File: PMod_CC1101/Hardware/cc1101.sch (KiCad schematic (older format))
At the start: 17 parts

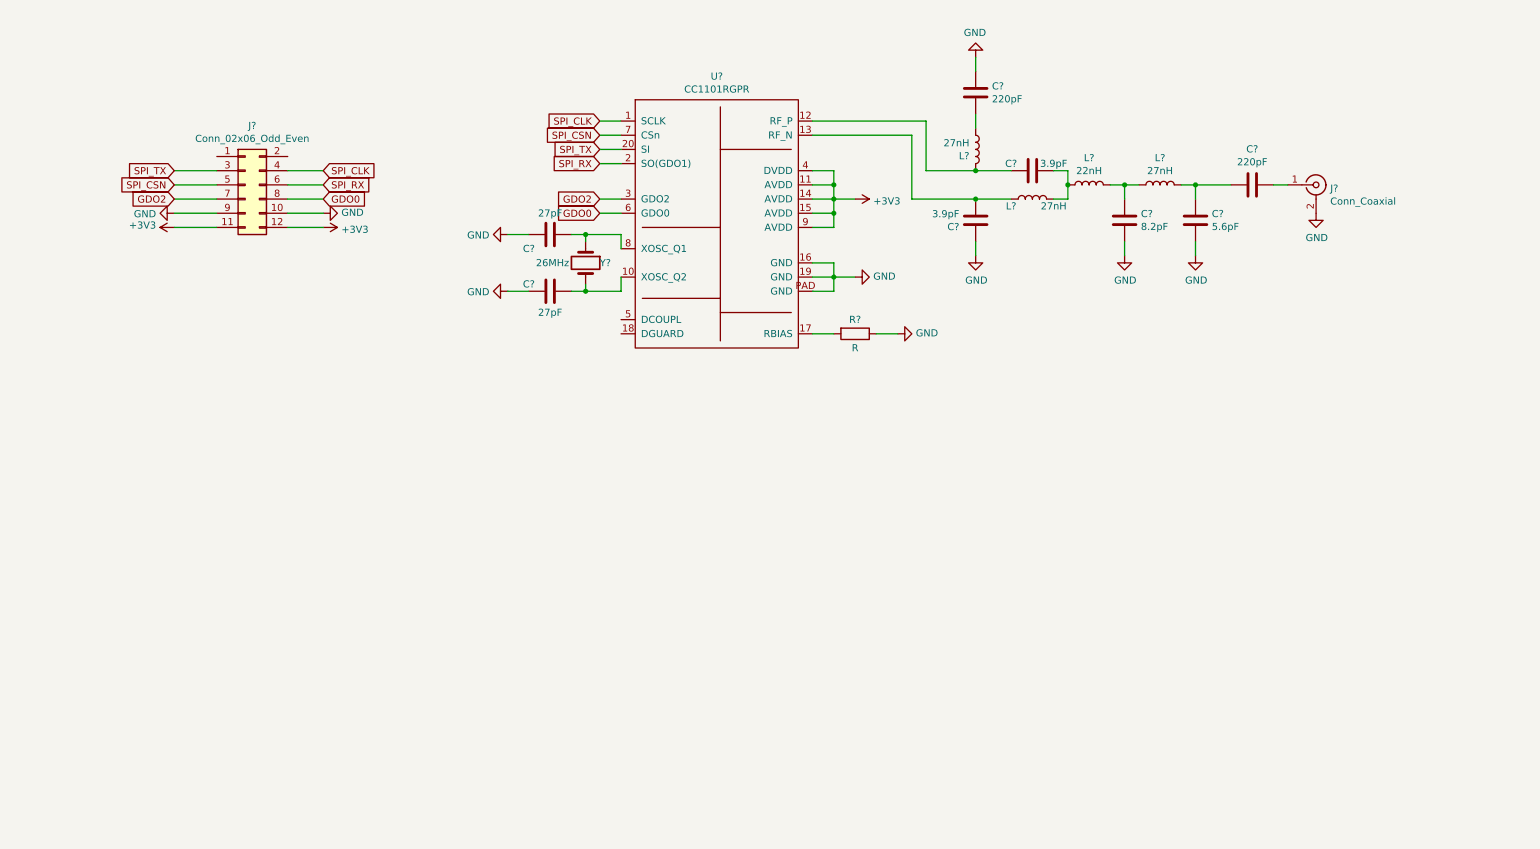
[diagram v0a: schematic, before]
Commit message: update the layout of the schematic
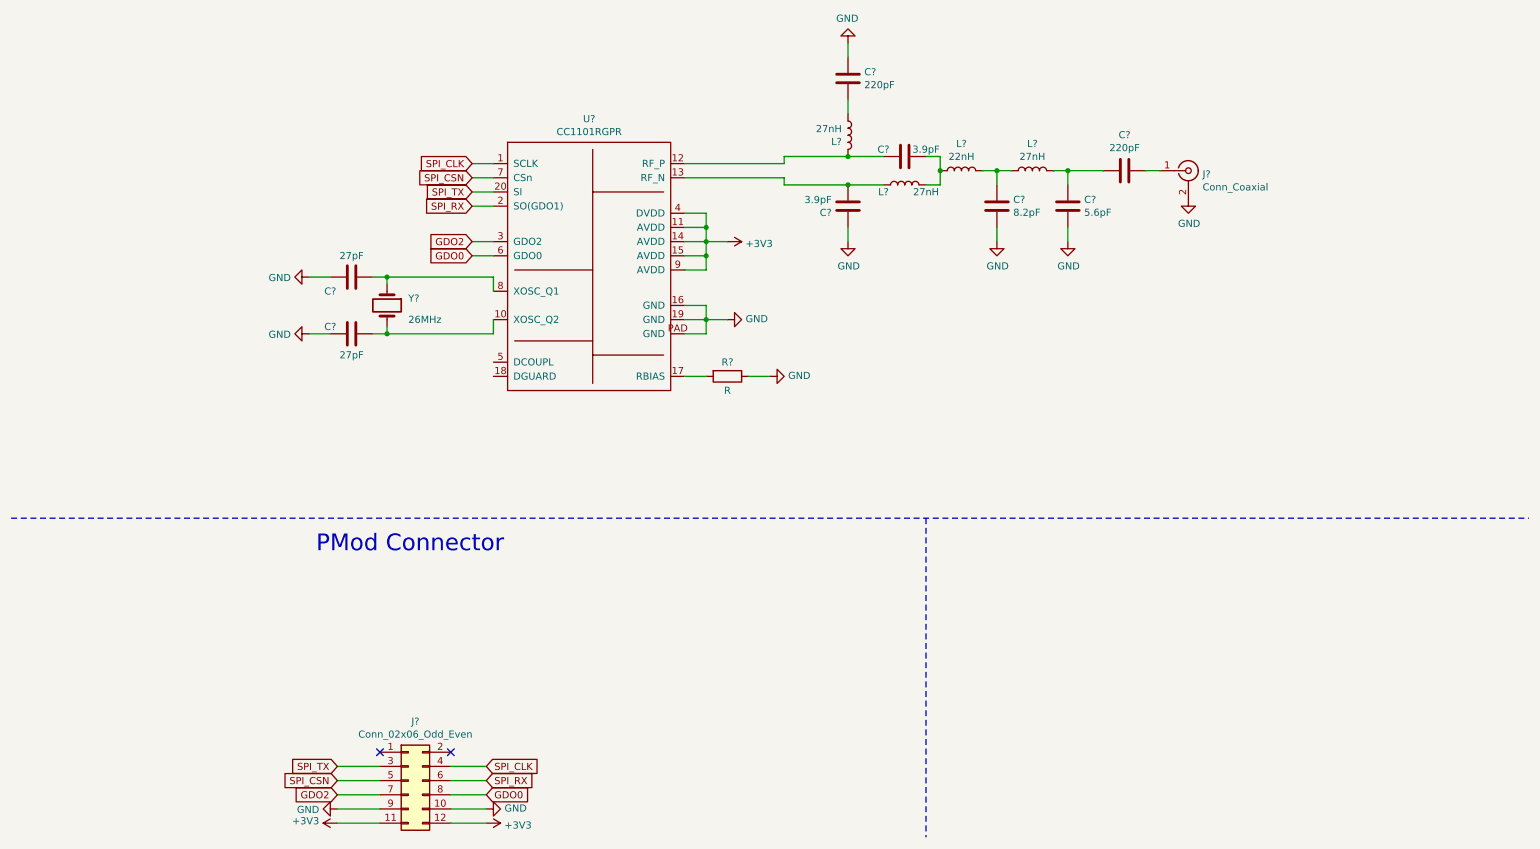
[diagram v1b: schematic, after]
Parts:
- J?: footprint (none) -> Connector_PinHeader_2.54mm:PinHeader_2x06_P2.54mm_Vertical
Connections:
- no-connect marks 0 -> 2
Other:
- note added: "PMod Connector"
- moved on the sheet: C?, J?, L?, R?, U?, Y?

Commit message: update the reference values and add a suitable crystal
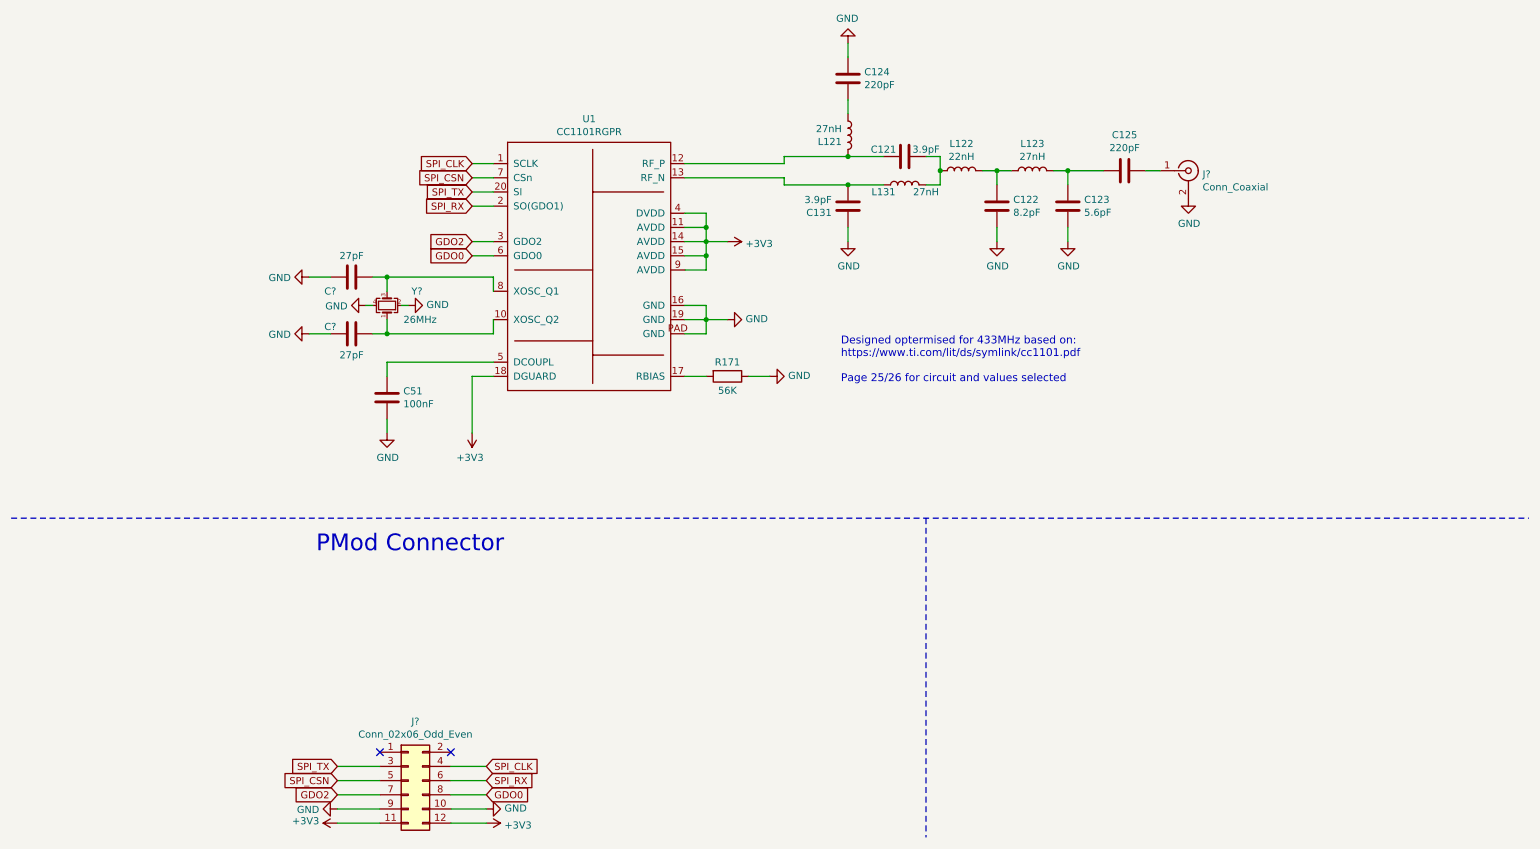
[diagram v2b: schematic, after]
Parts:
- removed Y?: 26MHz, symbol Device:Crystal
- added C51: 100nF, Capacitor_SMD:C_0603_1608Metric, symbol Device:C
- added Y?: 26MHz, Crystal:Crystal_SMD_Abracon_ABM3C-4Pin_5.0x3.2mm, symbol Device:Crystal_GND24_Small
- R171: renamed from R?; value R -> 56K; footprint (none) -> Resistor_SMD:R_0603_1608Metric
- gave numbers to parts that had none: 11
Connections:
- net +3V3: now also U1.18 (DGUARD)
- net GND: now also C51.1, Y?.2, Y?.4
- net at C?.2, U1.10 (XOSC_Q2): now also Y?.1
- net at U1.5 (DCOUPL): now also C51.2
- net at C?.1, U1.8 (XOSC_Q1): now also Y?.3
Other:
- note added: "Designed optermised for 433MHz based on:\nhttps://www.ti.com/lit/ds/symlink/cc1101.pdf\n\nPage 25/26 for circuit and values selected \n"
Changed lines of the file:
@@
 $EndComp
 $Comp
-L Device:C C?
+L Device:C C125
 U 1 1 60A35692
 P 8350 1850
-F 0 "C?" V 8098 1850 50  0000 C CNN
+F 0 "C125" V 8098 1850 50  0000 C CNN
 F 1 "220pF" V 8189 1850 50  0000 C CNN
 F 2 "Capacitor_SMD:C_0603_1608Metric" H 8388 1700 50  0001 C CNN
@@
 $EndComp
 $Comp
-L Device:C C?
+L Device:C C123
 U 1 1 60A35E36
 P 7950 2100
-F 0 "C?" H 8065 2146 50  0000 L CNN
+F 0 "C123" H 8065 2146 50  0000 L CNN
 F 1 "5.6pF" H 8065 2055 50  0000 L CNN
 F 2 "Capacitor_SMD:C_0603_1608Metric" H 7988 1950 50  0001 C CNN
@@
 $EndComp
 $Comp
-L Device:C C?
+L Device:C C122
 U 1 1 60A36923
 P 7450 2100
-F 0 "C?" H 7565 2146 50  0000 L CNN
+F 0 "C122" H 7565 2146 50  0000 L CNN
 F 1 "8.2pF" H 7565 2055 50  0000 L CNN
 F 2 "Capacitor_SMD:C_0603_1608Metric" H 7488 1950 50  0001 C CNN
@@
 $EndComp
 $Comp
-L Device:C C?
+L Device:C C121
 U 1 1 60A36D2F
 P 6800 1750
-F 0 "C?" V 6750 1600 50  0000 C CNN
+F 0 "C121" V 6750 1600 50  0000 C CNN
 F 1 "3.9pF" V 6750 1900 50  0000 C CNN
 F 2 "Capacitor_SMD:C_0603_1608Metric" H 6838 1600 50  0001 C CNN
@@
 $EndComp
 $Comp
-L Device:C C?
+L Device:C C131
 U 1 1 60A3755B
 P 6400 2100
-F 0 "C?" H 6515 2146 50  0000 L CNN
+F 0 "C131" H 6515 2146 50  0000 L CNN
 F 1 "3.9pF" H 6515 2055 50  0000 L CNN
 F 2 "" H 6438 1950 50  0001 C CNN
@@
 $EndComp
 $Comp
-L Device:C C?
+L Device:C C124
 U 1 1 60A37995
 P 6400 1200
-F 0 "C?" H 6285 1154 50  0000 R CNN
+F 0 "C124" H 6285 1154 50  0000 R CNN
 F 1 "220pF" H 6285 1245 50  0000 R CNN
 F 2 "Capacitor_SMD:C_0603_1608Metric" H 6438 1050 50  0001 C CNN
@@
 $EndComp
 $Comp
-L Device:L L?
+L Device:L L121
 U 1 1 60A38065
 P 6400 1600
-F 0 "L?" H 6356 1554 50  0000 R CNN
+F 0 "L121" H 6356 1554 50  0000 R CNN
 F 1 "27nH" H 6356 1645 50  0000 R CNN
 F 2 "Inductor_SMD:L_0603_1608Metric" H 6400 1600 50  0001 C CNN
@@
 $EndComp
 $Comp
-L Device:L L?
+L Device:L L131
 U 1 1 60A38A26
 P 6800 1950
-F 0 "L?" V 6750 2100 50  0000 C CNN
+F 0 "L131" V 6750 2100 50  0000 C CNN
 F 1 "27nH" V 6750 1800 50  0000 C CNN
 F 2 "Inductor_SMD:L_0603_1608Metric" H 6800 1950 50  0001 C CNN
@@
 $EndComp
 $Comp
-L Device:L L?
+L Device:L L122
 U 1 1 60A39321
 P 7200 1850
-F 0 "L?" V 7390 1850 50  0000 C CNN
+F 0 "L122" V 7390 1850 50  0000 C CNN
 F 1 "22nH" V 7299 1850 50  0000 C CNN
 F 2 "Inductor_SMD:L_0603_1608Metric" H 7200 1850 50  0001 C CNN
@@
 $EndComp
 $Comp
-L Device:L L?
+L Device:L L123
 U 1 1 60A3A077
 P 7700 1850
-F 0 "L?" V 7890 1850 50  0000 C CNN
+F 0 "L123" V 7890 1850 50  0000 C CNN
 F 1 "27nH" V 7799 1850 50  0000 C CNN
 F 2 "Inductor_SMD:L_0603_1608Metric" H 7700 1850 50  0001 C CNN
@@
 	6400 2250 6400 2350
 $Comp
-L JJH_Library:CC1101RGPR U?
+L JJH_Library:CC1101RGPR U1
 U 1 1 60A502FE
 P 4600 1900
-F 0 "U?" H 4575 2315 50  0000 C CNN
+F 0 "U1" H 4575 2315 50  0000 C CNN
 F 1 "CC1101RGPR" H 4575 2224 50  0000 C CNN
 F 2 "" H 4250 1900 50  0001 C CNN
@@
 	0    1    1    0
 $EndComp
-$Comp
-L Device:Crystal Y?
-U 1 1 60A6E09E
-P 3150 2800
-F 0 "Y?" V 3100 2950 50  0000 L CNN
-F 1 "26MHz" V 3250 2950 50  0000 L CNN
-F 2 "" H 3150 2800 50  0001 C CNN
-F 3 "~" H 3150 2800 50  0001 C CNN
-	1    3150 2800
-	0    1    1    0
-$EndComp
 Wire Wire Line
 	3900 2700 3900 2600
-Wire Wire Line
-	3150 2650 3150 2600
 Connection ~ 3150 2600
 Wire Wire Line
@@
 Wire Wire Line
 	3050 3000 3150 3000
-Wire Wire Line
-	3150 3000 3150 2950
 Wire Wire Line
 	3900 2900 3900 3000
@@
 	3750 1800 3900 1800
 $Comp
-L Device:R R?
+L Device:R R171
 U 1 1 60A8D230
 P 5550 3300
-F 0 "R?" V 5450 3300 50  0000 C CNN
-F 1 "R" V 5650 3300 50  0000 C CNN
-F 2 "" V 5480 3300 50  0001 C CNN
+F 0 "R171" V 5450 3300 50  0000 C CNN
+F 1 "56K" V 5650 3300 50  0000 C CNN
+F 2 "Resistor_SMD:R_0603_1608Metric" V 5480 3300 50  0001 C CNN
 F 3 "~" H 5550 3300 50  0001 C CNN
 	1    5550 3300
@@
 NoConn ~ 3600 5950
 NoConn ~ 3100 5950
+$Comp
+L Device:C C51
+U 1 1 60E263E0
+P 3150 3450
+F 0 "C51" H 3035 3404 50  0000 R CNN
+F 1 "100nF" H 3035 3495 50  0000 R CNN
+F 2 "Capacitor_SMD:C_0603_1608Metric" H 3188 3300 50  0001 C CNN
+F 3 "~" H 3150 3450 50  0001 C CNN
+	1    3150 3450
+	-1   0    0    1
+$EndComp
+Wire Wire Line
+	3150 3300 3150 3200
+Wire Wire Line
+	3150 3200 3900 3200
+$Comp
+L power:GND #PWR?
+U 1 1 60E2AE47
+P 3150 3700
+F 0 "#PWR?" H 3150 3450 50  0001 C CNN
+F 1 "GND" H 3155 3527 50  0000 C CNN
+F 2 "" H 3150 3700 50  0001 C CNN
+F 3 "" H 3150 3700 50  0001 C CNN
+	1    3150 3700
+	1    0    0    -1
+$EndComp
+$Comp
+L power:+3V3 #PWR?
+U 1 1 60E2B410
+P 3750 3700
+F 0 "#PWR?" H 3750 3550 50  0001 C CNN
+F 1 "+3V3" H 3765 3873 50  0000 C CNN
+F 2 "" H 3750 3700 50  0001 C CNN
+F 3 "" H 3750 3700 50  0001 C CNN
+	1    3750 3700
+	-1   0    0    1
+$EndComp
+Wire Wire Line
+	3750 3700 3750 3300
+Wire Wire Line
+	3750 3300 3900 3300
+Wire Wire Line
+	3150 3700 3150 3600
+Text Notes 6350 3350 0    55   ~ 0
+Designed optermised for 433MHz based on:\nhttps://www.ti.com/lit/ds/symlink/cc1101.pdf\n\nPage 25/26 for circuit and values selected \n
+$Comp
+L Device:Crystal_GND24_Small Y?
+U 1 1 60E33551
+P 3150 2800
+F 0 "Y?" V 3250 2550 50  0000 L CNN
+F 1 "26MHz" V 3050 2450 50  0000 L CNN
+F 2 "Crystal:Crystal_SMD_Abracon_ABM3C-4Pin_5.0x3.2mm" H 3150 2800 50  0001 C CNN
+F 3 "https://www.mouser.co.uk/datasheet/2/3/abrcs02719_1-2258580.pdf" H 3150 2800 50  0001 C CNN
+F 4 "815-ABM3C-26-D4YT" H 3150 2800 50  0001 C CNN "Mouser No."
+	1    3150 2800
+	0    -1   -1   0
+$EndComp
+Wire Wire Line
+	3150 2600 3150 2700
+Wire Wire Line
+	3150 2900 3150 3000
+$Comp
+L power:GND #PWR?
+U 1 1 60E3F2C7
+P 3000 2800
+F 0 "#PWR?" H 3000 2550 50  0001 C CNN
+F 1 "GND" V 3005 2672 50  0000 R CNN
+F 2 "" H 3000 2800 50  0001 C CNN
+F 3 "" H 3000 2800 50  0001 C CNN
+	1    3000 2800
+	0    1    1    0
+$EndComp
+$Comp
+L power:GND #PWR?
+U 1 1 60E3FC31
+P 3300 2800
+F 0 "#PWR?" H 3300 2550 50  0001 C CNN
+F 1 "GND" V 3305 2672 50  0000 R CNN
+F 2 "" H 3300 2800 50  0001 C CNN
+F 3 "" H 3300 2800 50  0001 C CNN
+	1    3300 2800
+	0    -1   -1   0
+$EndComp
+Wire Wire Line
+	3300 2800 3250 2800
+Wire Wire Line
+	3050 2800 3000 2800
 $EndSCHEMATC
